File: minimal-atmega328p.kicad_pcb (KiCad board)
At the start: 2 copper layers, 40 parts, among them J1 Conn_01x14_Male, J2 Conn_01x06_Male, J3 Conn_01x14_Male, SW1 SW_Push, U1 ATmega328P-PU, Y1 16MHz

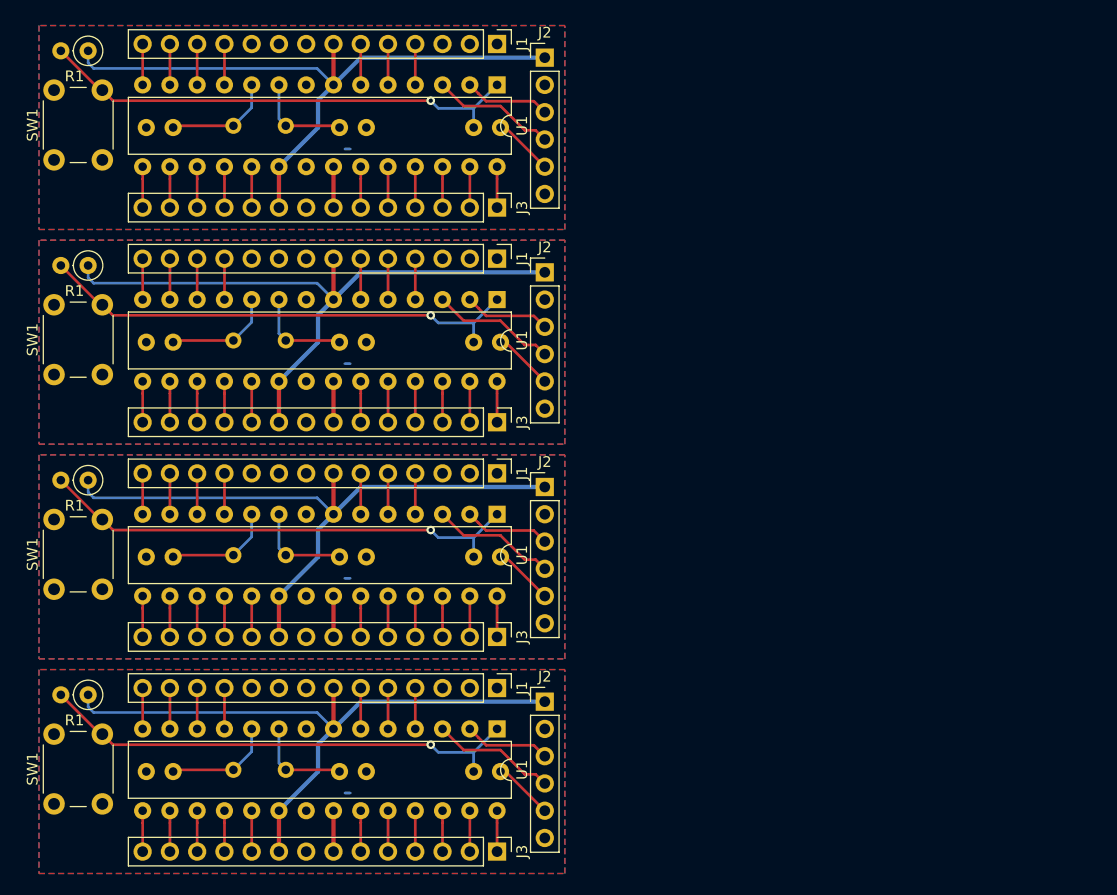
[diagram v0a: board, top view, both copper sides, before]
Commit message: update files
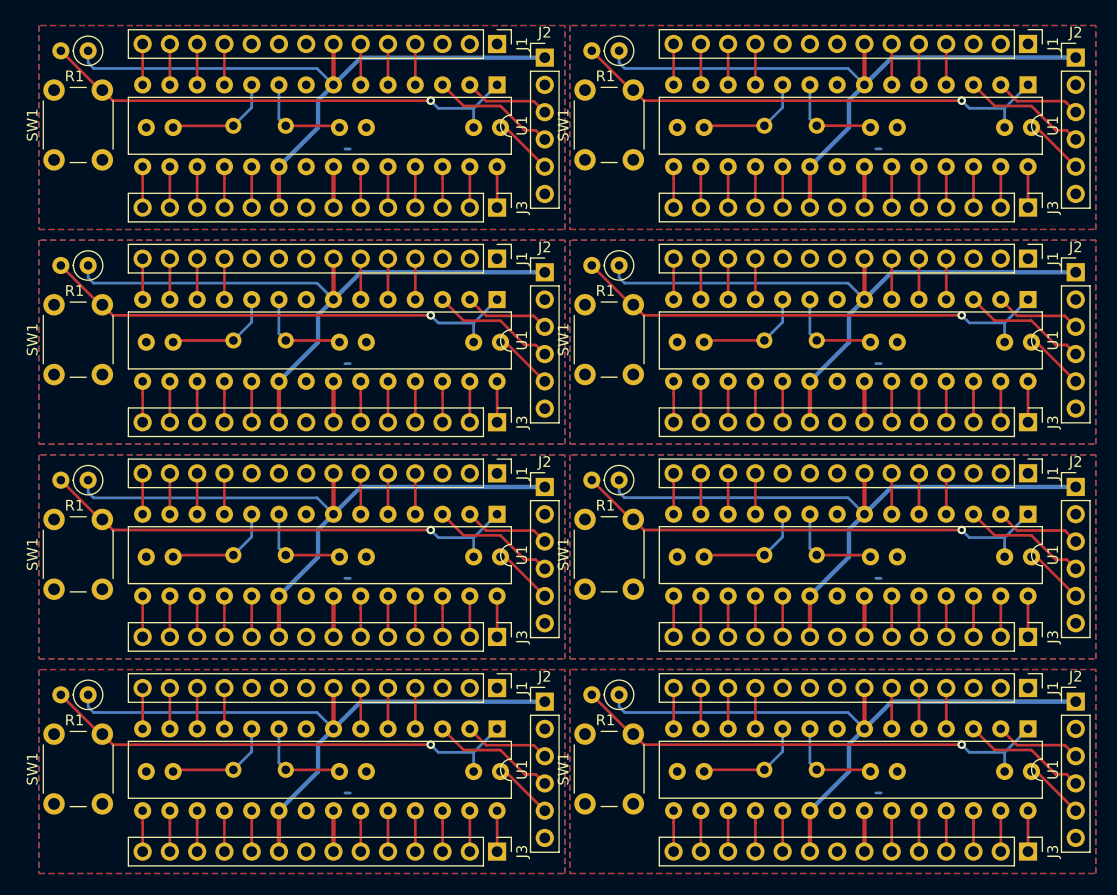
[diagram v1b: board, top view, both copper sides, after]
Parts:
- added C1: 22pF, Capacitor_THT:C_Disc_D3.8mm_W2.6mm_P2.50mm, B.Cu at (156.8, 117.1)
- added C1: 22pF, Capacitor_THT:C_Disc_D3.8mm_W2.6mm_P2.50mm, B.Cu at (156.8, 57.1)
- added C1: 22pF, Capacitor_THT:C_Disc_D3.8mm_W2.6mm_P2.50mm, B.Cu at (156.8, 97.1)
- added C1: 22pF, Capacitor_THT:C_Disc_D3.8mm_W2.6mm_P2.50mm, B.Cu at (156.8, 77.1)
- added C2: 22pF, Capacitor_THT:C_Disc_D3.8mm_W2.6mm_P2.50mm, B.Cu at (138.8, 117.1)
- added C2: 22pF, Capacitor_THT:C_Disc_D3.8mm_W2.6mm_P2.50mm, B.Cu at (138.8, 57.1)
- added C2: 22pF, Capacitor_THT:C_Disc_D3.8mm_W2.6mm_P2.50mm, B.Cu at (138.8, 77.1)
- added C2: 22pF, Capacitor_THT:C_Disc_D3.8mm_W2.6mm_P2.50mm, B.Cu at (138.8, 97.1)
- added C3: 0.1uF, Capacitor_THT:C_Disc_D3.8mm_W2.6mm_P2.50mm, B.Cu at (166.8, 117.1)
- added C3: 0.1uF, Capacitor_THT:C_Disc_D3.8mm_W2.6mm_P2.50mm, B.Cu at (166.8, 57.1)
- added C3: 0.1uF, Capacitor_THT:C_Disc_D3.8mm_W2.6mm_P2.50mm, B.Cu at (166.8, 97.1)
- added C3: 0.1uF, Capacitor_THT:C_Disc_D3.8mm_W2.6mm_P2.50mm, B.Cu at (166.8, 77.1)
- added J1: Conn_01x14_Male, Connector_PinHeader_2.54mm:PinHeader_1x14_P2.54mm_Vertical, F.Cu at (169.0, 109.3)
- added J1: Conn_01x14_Male, Connector_PinHeader_2.54mm:PinHeader_1x14_P2.54mm_Vertical, F.Cu at (169.0, 49.3)
- added J1: Conn_01x14_Male, Connector_PinHeader_2.54mm:PinHeader_1x14_P2.54mm_Vertical, F.Cu at (169.0, 89.3)
- added J1: Conn_01x14_Male, Connector_PinHeader_2.54mm:PinHeader_1x14_P2.54mm_Vertical, F.Cu at (169.0, 69.3)
- added J2: Conn_01x06_Male, Connector_PinHeader_2.54mm:PinHeader_1x06_P2.54mm_Vertical, F.Cu at (173.4, 110.6)
- added J2: Conn_01x06_Male, Connector_PinHeader_2.54mm:PinHeader_1x06_P2.54mm_Vertical, F.Cu at (173.4, 50.6)
- added J2: Conn_01x06_Male, Connector_PinHeader_2.54mm:PinHeader_1x06_P2.54mm_Vertical, F.Cu at (173.4, 90.6)
- added J2: Conn_01x06_Male, Connector_PinHeader_2.54mm:PinHeader_1x06_P2.54mm_Vertical, F.Cu at (173.4, 70.6)
- added J3: Conn_01x14_Male, Connector_PinHeader_2.54mm:PinHeader_1x14_P2.54mm_Vertical, F.Cu at (169.0, 124.5)
- added J3: Conn_01x14_Male, Connector_PinHeader_2.54mm:PinHeader_1x14_P2.54mm_Vertical, F.Cu at (169.0, 64.5)
- added J3: Conn_01x14_Male, Connector_PinHeader_2.54mm:PinHeader_1x14_P2.54mm_Vertical, F.Cu at (169.0, 84.5)
- added J3: Conn_01x14_Male, Connector_PinHeader_2.54mm:PinHeader_1x14_P2.54mm_Vertical, F.Cu at (169.0, 104.5)
- added R1: 10k, Resistor_THT:R_Axial_DIN0207_L6.3mm_D2.5mm_P2.54mm_Vertical, F.Cu at (130.9, 109.9)
- added R1: 10k, Resistor_THT:R_Axial_DIN0207_L6.3mm_D2.5mm_P2.54mm_Vertical, F.Cu at (130.9, 49.9)
- added R1: 10k, Resistor_THT:R_Axial_DIN0207_L6.3mm_D2.5mm_P2.54mm_Vertical, F.Cu at (130.9, 89.9)
- added R1: 10k, Resistor_THT:R_Axial_DIN0207_L6.3mm_D2.5mm_P2.54mm_Vertical, F.Cu at (130.9, 69.9)
- added SW1: SW_Push, Button_Switch_THT:SW_PUSH_6mm_H5mm, F.Cu at (127.7, 120.1)
- added SW1: SW_Push, Button_Switch_THT:SW_PUSH_6mm_H5mm, F.Cu at (127.7, 80.1)
- added SW1: SW_Push, Button_Switch_THT:SW_PUSH_6mm_H5mm, F.Cu at (127.7, 60.1)
- added SW1: SW_Push, Button_Switch_THT:SW_PUSH_6mm_H5mm, F.Cu at (127.7, 100.1)
- added U1: ATmega328P-PU, Package_DIP:DIP-28_W7.62mm, F.Cu at (169.0, 53.1)
- added U1: ATmega328P-PU, Package_DIP:DIP-28_W7.62mm, F.Cu at (169.0, 113.1)
- added U1: ATmega328P-PU, Package_DIP:DIP-28_W7.62mm, F.Cu at (169.0, 73.1)
- added U1: ATmega328P-PU, Package_DIP:DIP-28_W7.62mm, F.Cu at (169.0, 93.1)
- added Y1: 16MHz, Crystal:Crystal_HC49-4H_Vertical, B.Cu at (149.3, 56.9)
- added Y1: 16MHz, Crystal:Crystal_HC49-4H_Vertical, B.Cu at (149.3, 116.9)
- added Y1: 16MHz, Crystal:Crystal_HC49-4H_Vertical, B.Cu at (149.3, 96.9)
- added Y1: 16MHz, Crystal:Crystal_HC49-4H_Vertical, B.Cu at (149.3, 76.9)
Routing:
- net (no net): track 679.8 -> 1586.2 mm, vias 3 -> 7
